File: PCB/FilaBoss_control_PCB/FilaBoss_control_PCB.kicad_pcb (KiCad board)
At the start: 2 copper layers, 101.6 x 80 mm, 43 parts, among them J1 Encoder, J10 Power 3.3v, J11 SCL/SDA, J12 power 12v, J13 power 5v, J14 Fan connector, J15 power 12v, J16 Screen, J2 SPOOL, J3 PULLER, J4 RX/TX, J5 Barrel_Jack_SMD, J6 INA219, J7 Stepper, J8 limit switch, J9 Conn_01x04_Pot, Q1 IRLZ44N, Q2 IRLZ44N, U2 R-78E5.0-0.5, U4 R-78E12-2

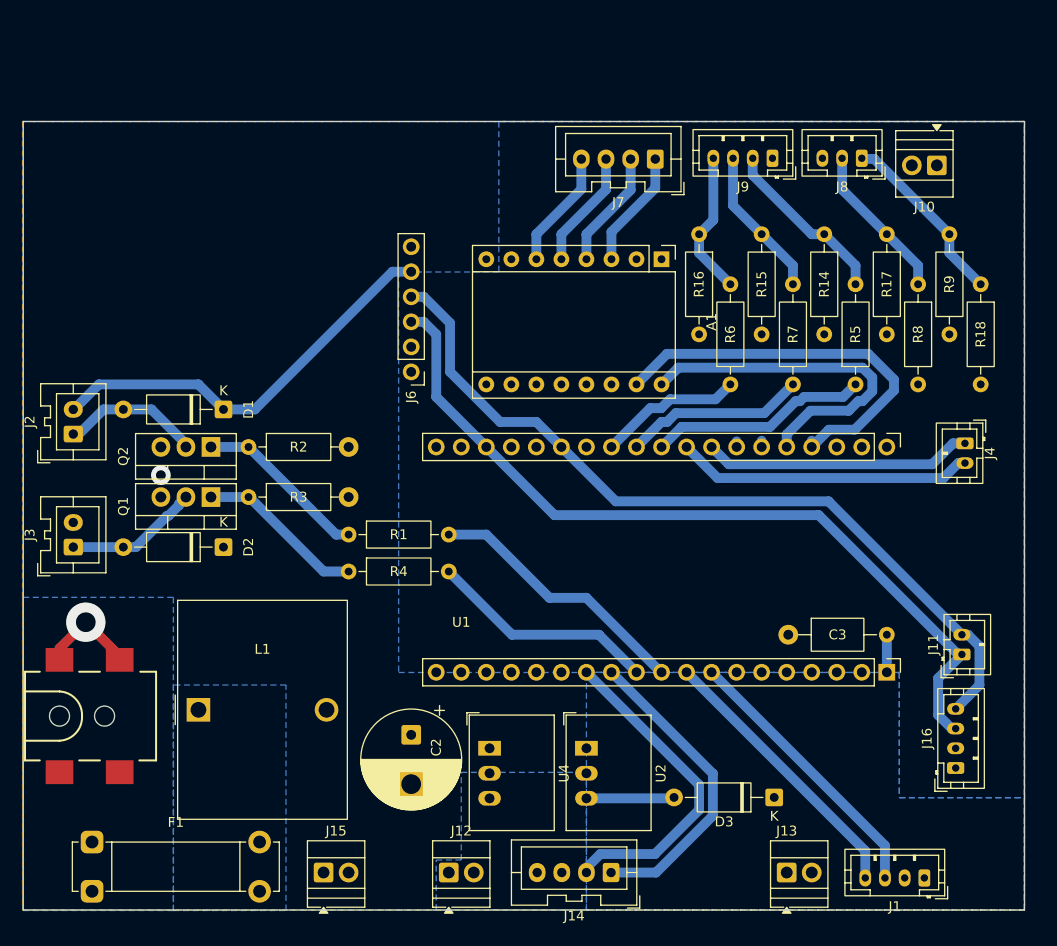
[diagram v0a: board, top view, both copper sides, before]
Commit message: pcb v2
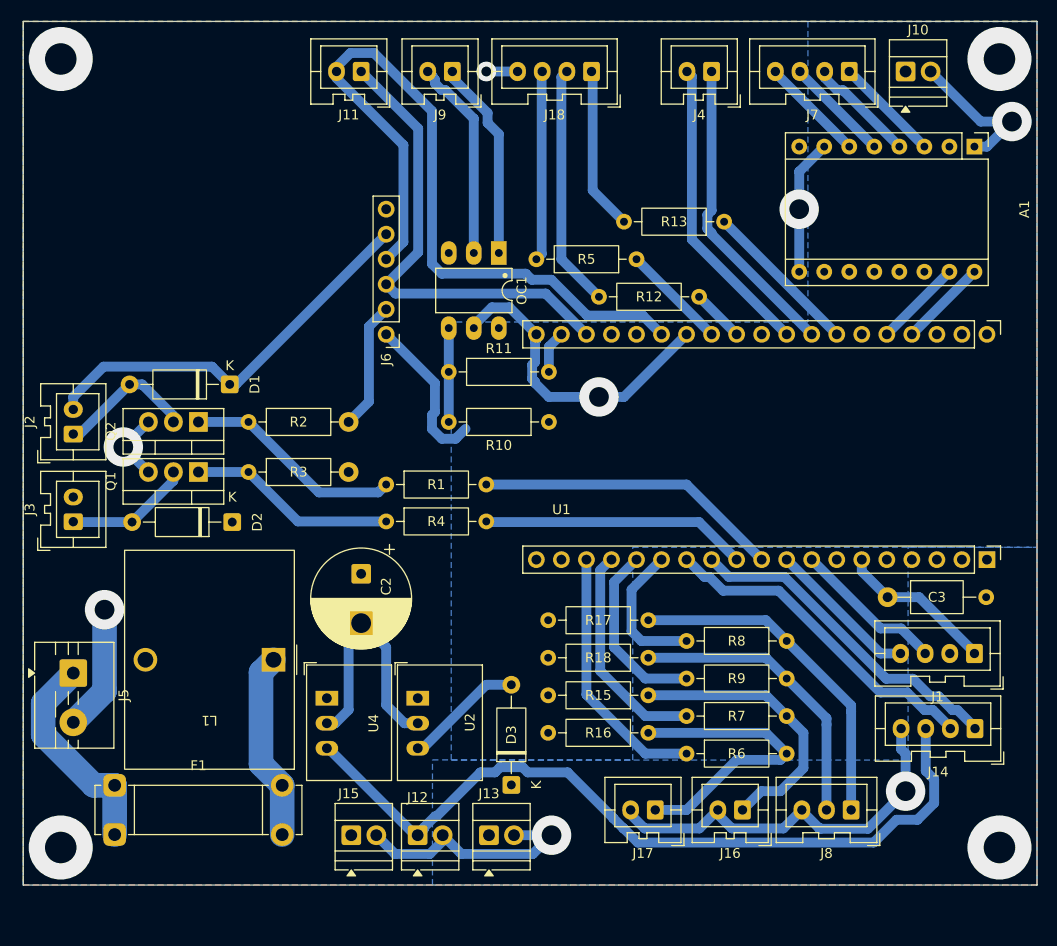
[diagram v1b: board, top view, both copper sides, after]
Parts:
- removed R14: 4.7k, Resistor_THT:R_Axial_DIN0207_L6.3mm_D2.5mm_P10.16mm_Horizontal
- added J17: manual, Connector_JST:JST_XA_B02B-XASK-1_1x02_P2.50mm_Vertical, F.Cu at (102.2, 166.4)
- added J18: Control leds, Connector_JST:JST_XA_B04B-XASK-1_1x04_P2.50mm_Vertical, F.Cu at (95.8, 91.4)
- added OC1: H11A1, PCM_Package_DIP_AKL:DIP-6_W7.62mm_LongPads, F.Cu at (86.4, 109.9)
- added R10: 4.7k, Resistor_THT:R_Axial_DIN0207_L6.3mm_D2.5mm_P10.16mm_Horizontal, F.Cu at (91.4, 127.0)
- added R11: 330R, Resistor_THT:R_Axial_DIN0207_L6.3mm_D2.5mm_P10.16mm_Horizontal, F.Cu at (81.3, 121.9)
- added R12: 220R, Resistor_THT:R_Axial_DIN0207_L6.3mm_D2.5mm_P10.16mm_Horizontal, F.Cu at (106.7, 114.3)
- added R13: 220R, Resistor_THT:R_Axial_DIN0207_L6.3mm_D2.5mm_P10.16mm_Horizontal, F.Cu at (109.2, 106.7)
- J1: footprint Connector_JST:JST_PH_B4B-PH-K_1x04_P2.00mm_Vertical -> Connector_JST:JST_XA_B04B-XASK-1_1x04_P2.50mm_Vertical
- J11: value SCL/SDA -> SDA/SCL; footprint Connector_JST:JST_PH_B2B-PH-K_1x02_P2.00mm_Vertical -> Connector_JST:JST_XA_B02B-XASK-1_1x02_P2.50mm_Vertical
- J15: value power 12v -> power 24v
- J16: value Screen -> Load; footprint Connector_JST:JST_PH_B4B-PH-K_1x04_P2.00mm_Vertical -> Connector_JST:JST_XA_B02B-XASK-1_1x02_P2.50mm_Vertical
- J4: value RX/TX -> Conn_01x02_Pin; footprint Connector_JST:JST_PH_B2B-PH-K_1x02_P2.00mm_Vertical -> Connector_JST:JST_XA_B02B-XASK-1_1x02_P2.50mm_Vertical
- J5: value Barrel_Jack_SMD -> Screw_Terminal_01x02_P5mm; footprint PCM_SparkFun-Connector:Barrel_Jack_SMD -> TerminalBlock:TerminalBlock_MaiXu_MX126-5.0-02P_1x02_P5.00mm
- J8: footprint Connector_JST:JST_PH_B3B-PH-K_1x03_P2.00mm_Vertical -> Connector_JST:JST_XA_B03B-XASK-1_1x03_P2.50mm_Vertical
- J9: value Conn_01x04_Pot -> Extruder; footprint Connector_JST:JST_PH_B4B-PH-K_1x04_P2.00mm_Vertical -> Connector_JST:JST_XA_B02B-XASK-1_1x02_P2.50mm_Vertical
- R5: value 100R -> 220R
- R6, R7, R8, R9: value 100R -> 330R
- moved J11 84.9 mm to (72.4, 91.4), turned to 180 degrees
- moved J8 66.1 mm to (122.1, 166.4)
- moved R16 50.9 mm to (101.5, 158.5), turned to 180 degrees
- moved R18 50.7 mm to (101.5, 150.9), turned to 180 degrees
- moved R15 48.2 mm to (101.5, 154.7), turned to 180 degrees
- moved R9 48.0 mm to (115.6, 153.0), turned to 180 degrees
- moved R17 46.0 mm to (101.5, 147.1), turned to 180 degrees
- moved J4 45.7 mm to (108.0, 91.4), turned to 180 degrees
- moved J14 39.7 mm to (134.7, 158.1)
- moved R8 38.6 mm to (115.6, 149.2), turned to 180 degrees
- moved R6 37.7 mm to (105.4, 160.7), turned to 0 degrees
- moved R7 35.3 mm to (105.4, 156.8), turned to 0 degrees
- moved A1 33.7 mm to (134.6, 99.1)
- moved J9 33.7 mm to (81.6, 91.4)
- moved J13 30.4 mm to (85.4, 168.9)
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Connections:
- J10 pad 1: GND -> +3.3V
- J10 pad 2: +3.3V -> GND
- J16 pad 1: GND -> Net-(J16--)
- J16 pad 2: +3.3V -> GND
- J9 pad 1: GND -> Net-(J9--)
- J9 pad 2: Net-(J9-Pin_2) -> Net-(J9-+)
- R15 pad 1: Net-(J9-Pin_3) -> Net-(J16--)
- R16 pad 1: Net-(J9-Pin_4) -> Net-(J17--)
- R17 pad 1: Net-(J8-Pad2) -> Net-(J8-Pad1)
- R18 pad 1: Net-(J8-Pad1) -> Net-(J8-Pad2)
- R5 pad 1: Net-(U1-GPIO5) -> Net-(U1-GPIO19)
- R5 pad 2: Net-(J9-Pin_2) -> Net-(J18-Pin_3)
- R6 pad 1: Net-(U1-GPIO19) -> Net-(U1-GPIO36)
- R6 pad 2: Net-(J9-Pin_4) -> Net-(J17--)
- R7 pad 1: Net-(U1-GPIO18) -> Net-(U1-GPIO39)
- R7 pad 2: Net-(J9-Pin_3) -> Net-(J16--)
- R8 pad 1: Net-(J8-Pad2) -> Net-(J8-Pad1)
- R9 pad 1: Net-(J8-Pad1) -> Net-(J8-Pad2)
- U1 pad 16: unconnected-(U1-GPIO39-Pad16) -> Net-(U1-GPIO39)
- U1 pad 17: unconnected-(U1-GPIO36-Pad17) -> Net-(U1-GPIO36)
- U1 pad 23: Net-(A1-STEP) -> Net-(A1-DIR)
- U1 pad 24: Net-(A1-DIR) -> Net-(A1-STEP)
- U1 pad 26: unconnected-(U1-GPIO4-Pad26) -> Net-(U1-GPIO4)
- U1 pad 29: Net-(U1-GPIO5) -> unconnected-(U1-GPIO5-Pad29)
- U1 pad 37: unconnected-(U1-GPIO23-Pad37) -> Net-(U1-GPIO23)
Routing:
- net GND: track 0.00 -> 205.3 mm, vias 1 -> 8
- net +12V: track 0.00 -> 81.5 mm
- net Net-(J11--): track 83.1 -> 47.8 mm
- net Net-(A1-STEP): track 41.0 -> 8.98 mm
- net Net-(J17--): track 0.00 -> 30.6 mm
- net Net-(J16--): track 0.00 -> 28.8 mm
- net Net-(A1-DIR): track 36.4 -> 8.98 mm
- net Net-(U1-GPIO36): track 0.00 -> 26.3 mm
- net Net-(J18-Pin_2): track 0.00 -> 24.7 mm
- net Net-(U1-GPIO39): track 0.00 -> 22.5 mm
- net Net-(U1-GPIO5): track 22.3 -> 0.00 mm
- net Net-(J9-+): track 0.00 -> 20.6 mm
- net Net-(J9--): track 0.00 -> 20.4 mm
- net Net-(J18-Pin_3): track 0.00 -> 19.3 mm
- net VDC: track 0.00 -> 19.2 mm
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- removed copper zone on B.Cu, net +12V
- removed copper zone on B.Cu, net LINE
- removed copper zone on B.Cu, net VDC
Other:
- board size 101.6 x 80 mm -> 102.9 x 87.6 mm
